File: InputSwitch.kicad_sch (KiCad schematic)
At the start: 10 parts, among them SW401 RotaryEncoder, SW402 SW_UP, SW403 SW_DOWN, SW404 SW_LEFT, SW405 SW_RIGHT, SW406 SW_ENTER, U401 74HC14

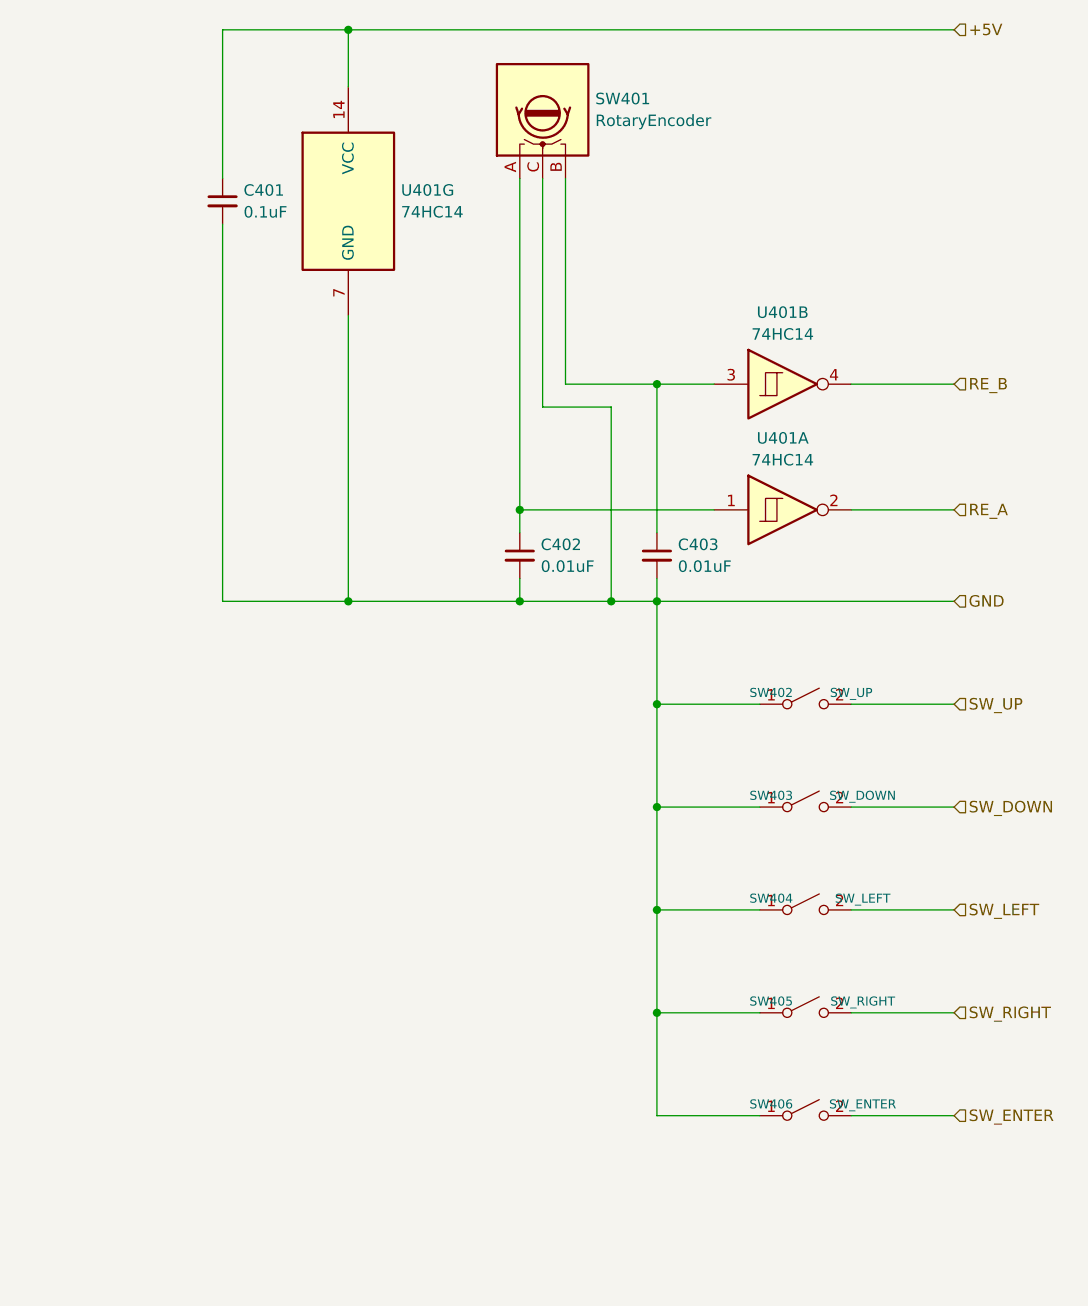
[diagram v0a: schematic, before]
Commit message: 途中
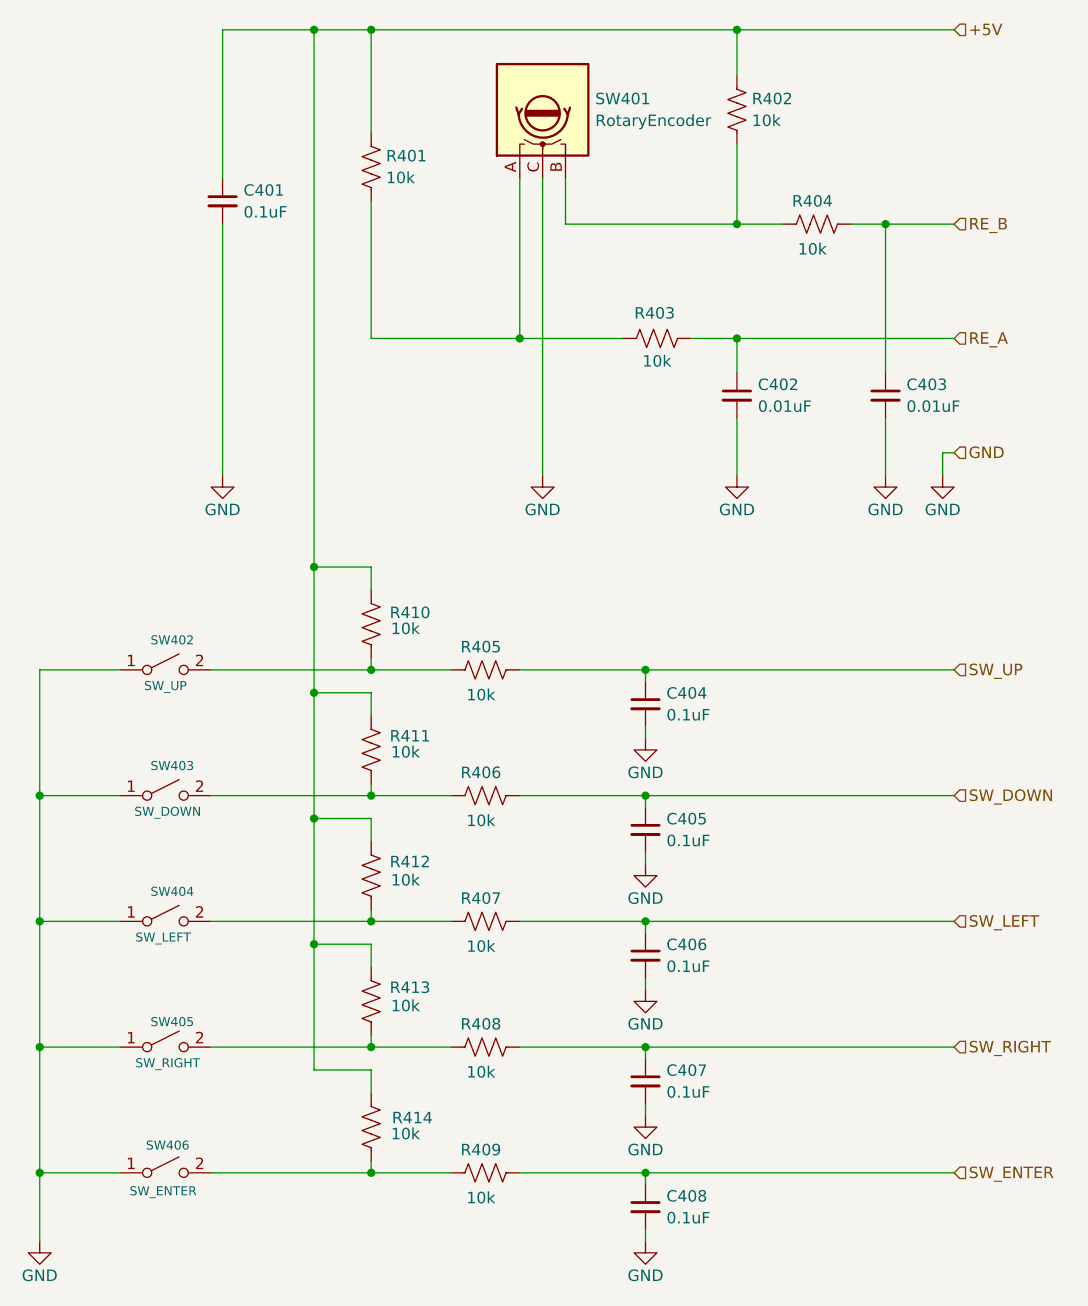
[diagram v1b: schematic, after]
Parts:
- removed U401: 74HC14, Package_DIP:DIP-14_W7.62mm_LongPads, symbol 74xx:74HC14
- added C404, C405, C406, C407, C408: 0.1uF, Capacitor_THT:C_Disc_D3.0mm_W2.0mm_P2.50mm, symbol Device:C_Small
- added R401, R402, R403, R404, R405, R406, R407, R408, R409, R410, R411, R412, R413, R414: 10k, symbol Device:R_US
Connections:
- net +5V: now also R401.1, R402.1, R410.2, R411.2, R412.2, R413.2, R414.2
- net GND: now also C404.2, C405.2, C406.2, C407.2, C408.2
- net RE_A: now also C402.1, R403.2
- net RE_B: now also C403.1, R404.2
- net SW_DOWN: now also C405.1, R406.2; no longer SW403.2 (B)
- net SW_ENTER: now also C408.1, R409.2; no longer SW406.2 (B)
- net SW_LEFT: now also C406.1, R407.2; no longer SW404.2 (B)
- net SW_RIGHT: now also C407.1, R408.2; no longer SW405.2 (B)
- net SW_UP: now also C404.1, R405.2; no longer SW402.2 (B)
- net at SW401.A: now also R401.2, R403.1; no longer C402.1
- net at SW401.B: now also R402.2, R404.1; no longer C403.1
- new net: R408.1, R413.1, SW405.2 (B)
- new net: R407.1, R412.1, SW404.2 (B)
- new net: R406.1, R411.1, SW403.2 (B)
- new net: R409.1, R414.1, SW406.2 (B)
- new net: R405.1, R410.1, SW402.2 (B)
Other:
- moved on the sheet: C402, C403, SW402, SW403, SW404, SW405, SW406
